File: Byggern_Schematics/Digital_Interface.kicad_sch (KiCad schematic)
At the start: 12 parts, among them IC6 MAX233, J2 Conn_02x05_Odd_Even, J5 DE9_Socket, U3 MCP2515-xSO, U4 MCP2551-I-P, Y3 16MHz

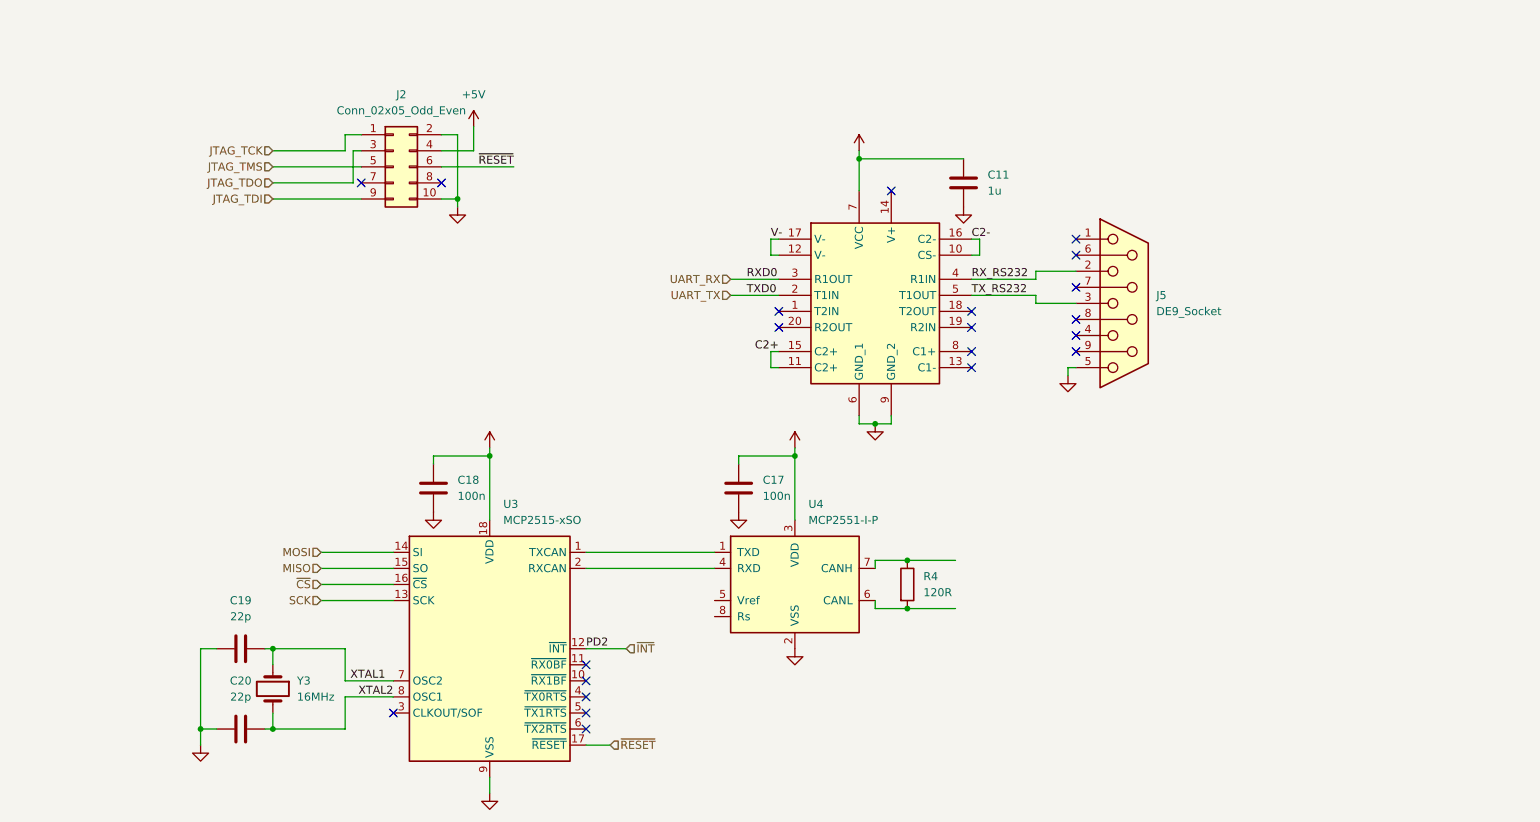
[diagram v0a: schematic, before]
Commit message: Finnished schematic
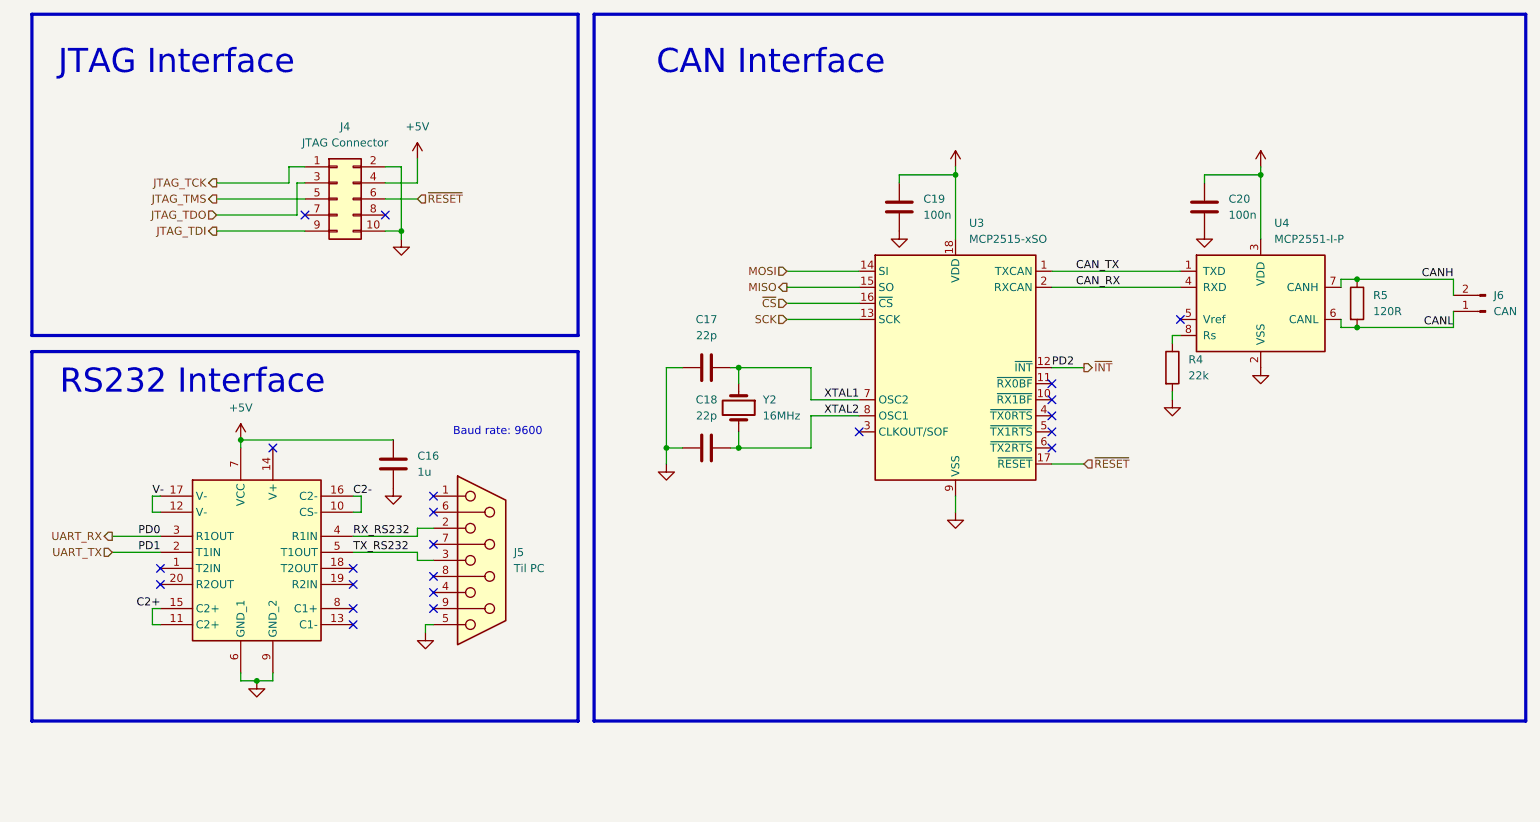
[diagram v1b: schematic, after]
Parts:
- added J6: CAN, symbol Connector:Conn_01x02_Pin
- added R4: 22k, symbol Device:R
- J4: renamed from J2; value Conn_02x05_Odd_Even -> JTAG Connector
- J5: value DE9_Socket -> Til PC
- renumbered C11 to C16, C19 to C17, C20 to C18, C18 to C19, C17 to C20, IC6 to IC5, R4 to R5, Y3 to Y2
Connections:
- net GND: now also R4.2
- net CAN_TX: now reaches U3.1 (TXCAN), U4.1 (TXD)
- net CAN_RX: now reaches U3.2 (RXCAN), U4.4 (RXD)
- net CANH: now reaches R5.1, U4.7 (CANH)
- net CANH: now also J6.2 (Pin_2)
- net CANL: now reaches R5.2, U4.6 (CANL)
- net CANL: now also J6.1 (Pin_1)
- net at U4.8 (Rs): now also R4.1
- no-connect marks 21 -> 22
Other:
- note added: "Baud rate: 9600"
- note added: "CAN Interface"
- note added: "JTAG Interface"
- note added: "RS232 Interface"
- company: (none) -> Gruppe 31
- title: (none) -> Veldig pent yup yup
- moved on the sheet: C16, C17, C18, C19, C20, J4, J5, R5, U3, U4, Y2
